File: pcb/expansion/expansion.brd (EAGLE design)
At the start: 88 x 42 mm, 46 parts, among them IC3 STM32F042F4, J1 AUDIO_JACK_3.5MM_PTH, J2 AUDIO_JACK_3.5MM_PTH, J3 AUDIO_JACK_3.5MM_PTH, J4 AUDIO_JACK_3.5MM_PTH, J5 AUDIO_JACK_3.5MM_PTH, J6 AUDIO_JACK_3.5MM_PTH, SW3 324_SW, SW4 324_SW, U1 USBC_16P, U2 USBC_16P, U4 XC6206_DEV

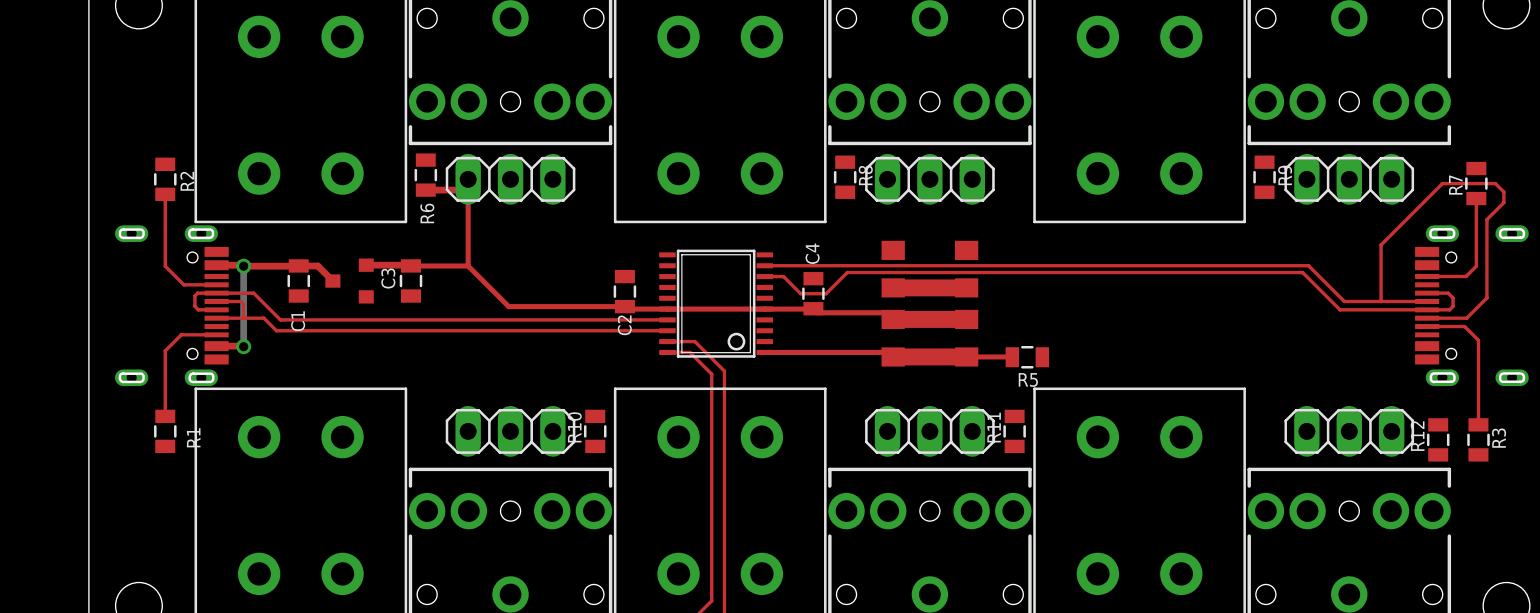
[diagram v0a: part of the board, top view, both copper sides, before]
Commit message: working on pcb
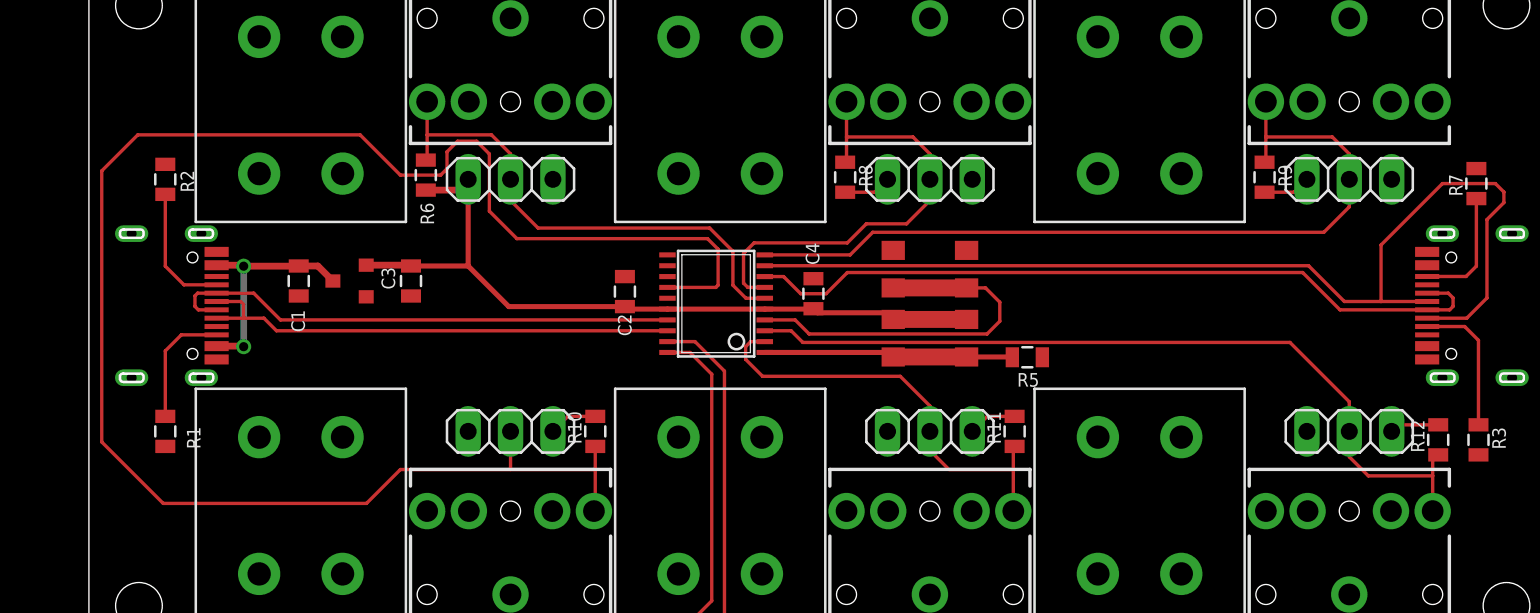
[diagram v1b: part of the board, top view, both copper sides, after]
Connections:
- net GND: now also JP6.3
- net N$3: now also IC3.6
- net N$4: now also IC3.7
- net N$6: now also IC3.10
- net N$7: now also IC3.14
- net N$8: now also IC3.2
- net N$9: now also IC3.3
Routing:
- net N$7: track 0.00 -> 104.6 mm
- net N$9: track 0.00 -> 49.1 mm
- net N$6: track 0.00 -> 48.5 mm
- net N$3: track 0.00 -> 30.7 mm
- net N$4: track 0.00 -> 27.5 mm
- net N$8: track 0.00 -> 26.3 mm
- net BUTTON1: track 4.40 -> 22.6 mm
- net +3V3: track 45.4 -> 59.3 mm
